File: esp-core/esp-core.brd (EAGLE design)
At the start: 35.6 x 35.6 mm, 9 parts

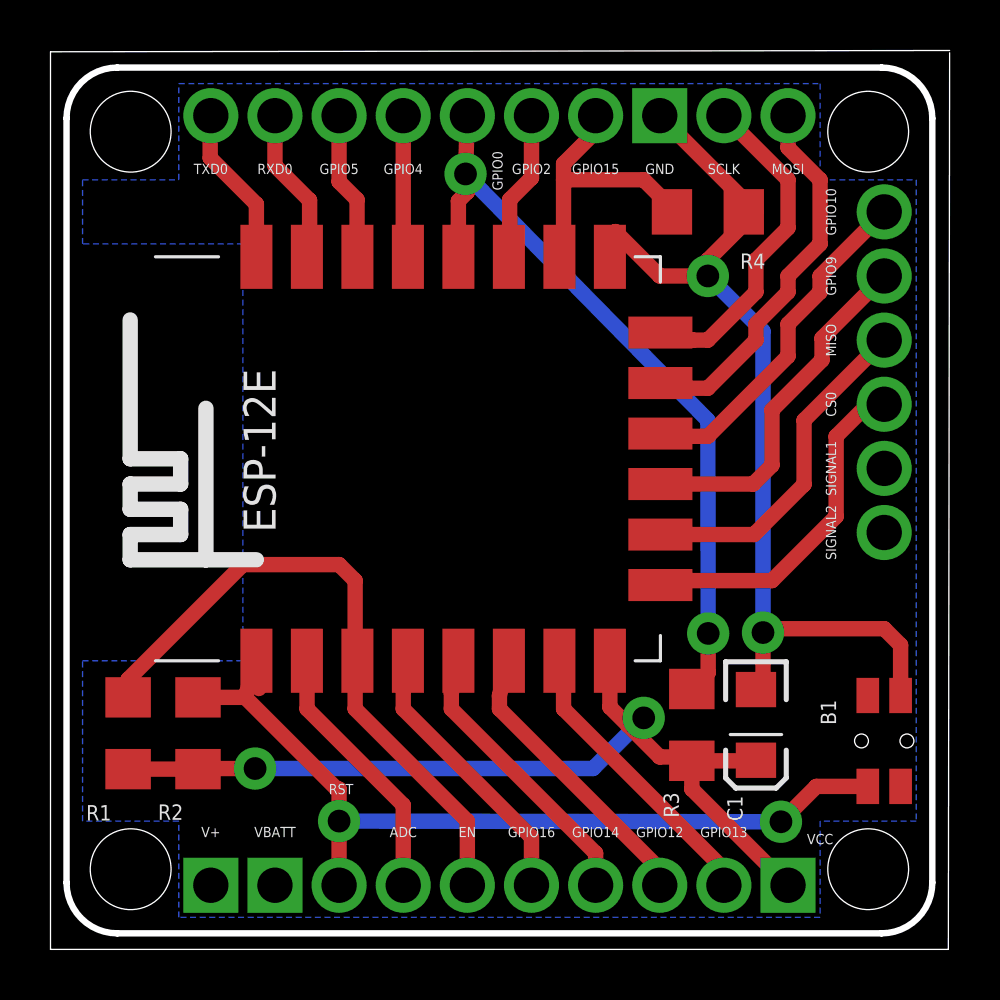
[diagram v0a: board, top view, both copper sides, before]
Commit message: core board fixes
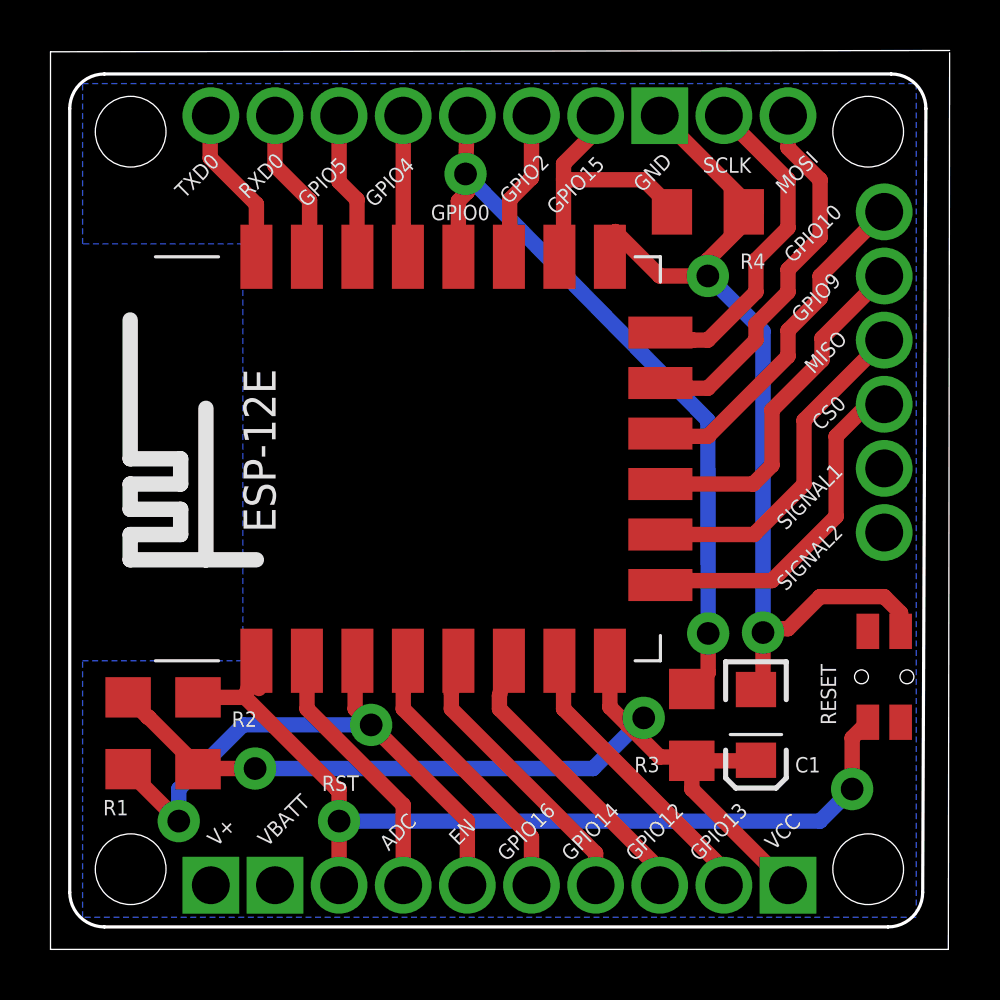
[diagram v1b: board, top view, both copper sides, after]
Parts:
- removed B1: (no value), ESPstack:SKSCLDE010
- added RESET: (no value), ESPstack:SKSCLDE010
- turned R1 to 90 degrees
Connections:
- net GND: now also RESET.1, RESET.2; no longer B1.1, B1.2
- net RESET: now also RESET.3, RESET.4; no longer B1.3, B1.4
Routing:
- net EN: track 27.6 -> 23.6 mm, vias 0 -> 2
- net RESET: track 35.0 -> 37.3 mm
- net GND: track 39.6 -> 38.9 mm
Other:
- outline, holes or cut-outs redrawn
